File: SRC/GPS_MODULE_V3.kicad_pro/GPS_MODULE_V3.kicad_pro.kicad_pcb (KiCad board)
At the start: 4 copper layers, 50.1 x 41 mm, 127 parts, among them J3 nano_sim, J4 Micro_SD_Card, J5 Conn_02x06_Counter_Clockwise, Q1 SSM3J328R-HXY, Q2 BSN20, Q3 BSN20, U1 SY8089AAAC, U2 STM32F103C8Tx, U3 A9G_MODULE, U4 MAX485E, U5 XC6206PxxxMR, U7 ATA6561-GAQW-N, U8 W25Q32JVSS, Y1 8MHz, Y2 32.678KHz

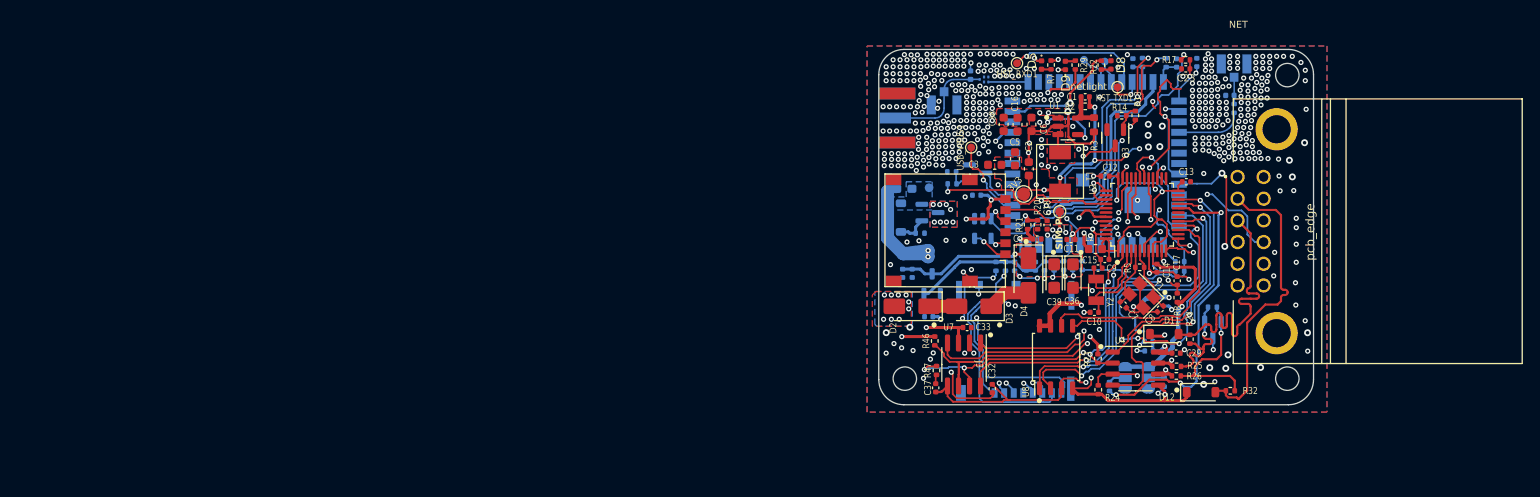
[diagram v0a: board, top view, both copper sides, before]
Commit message: GPS all files BOM and placemnt guide files added
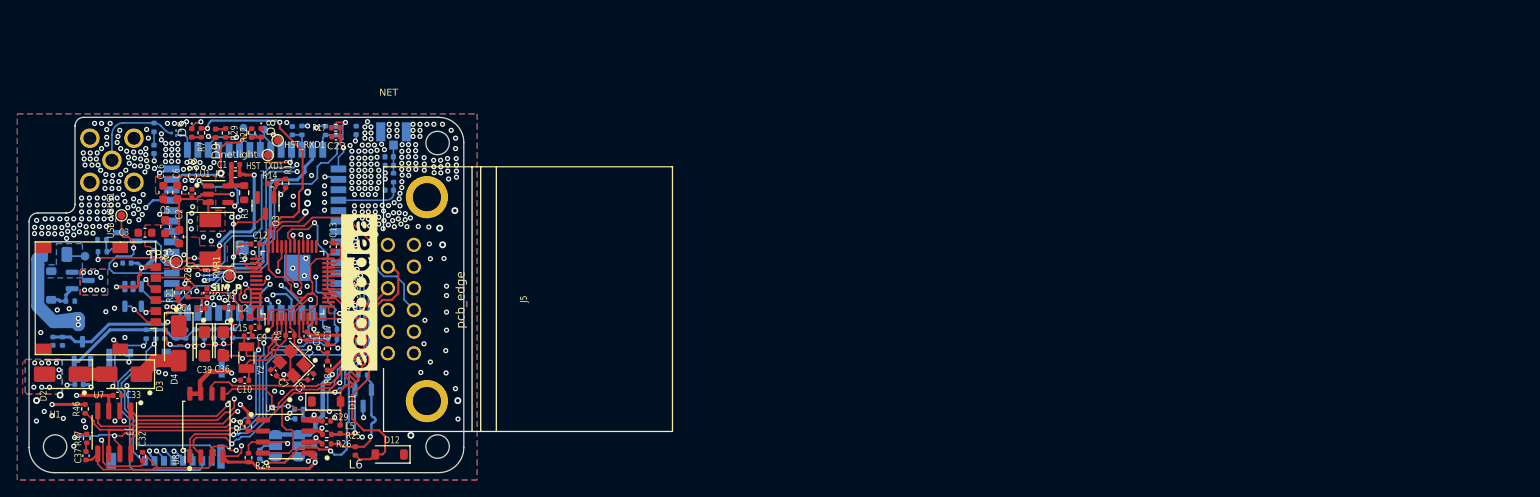
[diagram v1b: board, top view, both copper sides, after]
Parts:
- removed AE3: Antenna_Shield, greencharge-footprints:UFL_COAX_CONN23370191
- removed R32: 0R, Resistor_SMD:R_0402_1005Metric
- added C35: 100n, Capacitor_SMD:C_0402_1005Metric, B.Cu at (139.8, 89.6)
- added C40: C_Small, Capacitor_SMD:C_0402_1005Metric, B.Cu at (166.9, 82.2)
- added C41: C_Small, Capacitor_SMD:C_0402_1005Metric, B.Cu at (166.9, 79.4)
- added L5: L_Ferrite, Inductor_SMD:L_0402_1005Metric, F.Cu at (161.3, 109.8)
- added L6: L_Ferrite, Inductor_SMD:L_0402_1005Metric, F.Cu at (163.0, 112.3)
- AE1: footprint Connector_Coaxial:SMA_Samtec_SMA-J-P-X-ST-EM1_EdgeMount -> Connector_Coaxial:SMA_Molex_73251-2200_Horizontal
- C38: footprint Capacitor_SMD:C_0603_1608Metric -> Capacitor_SMD:C_0402_1005Metric
- G***: moved to F.Cu
- L2: footprint Inductor_SMD:L_0603_1608Metric -> Inductor_SMD:L_0402_1005Metric
- R28: value 0R -> 22R; moved to B.Cu
- TH1: footprint Fuse:Fuse_0603_1608Metric_Pad1.05x0.95mm_HandSolder -> Fuse:Fuse_1206_3216Metric
- TP2: footprint TestPoint:TestPoint_Pad_D1.5mm -> TestPoint:TestPoint_Pad_D1.0mm
- moved R28 121.8 mm to (139.8, 75.0)
- moved C16 98.8 mm to (140.9, 82.5)
- moved C6 98.8 mm to (142.5, 82.5)
- moved G*** 98.7 mm to (163.5, 94.0)
- moved C13 98.6 mm to (160.5, 88.7), turned to 90 degrees
- moved C23 98.2 mm to (160.8, 76.1)
- moved D10 98.2 mm to (163.9, 106.2)
- moved J5 98.2 mm to (182.4, 94.8)
- moved C12 98.2 mm to (151.5, 88.4)
- moved C14 98.2 mm to (157.5, 99.0)
- moved C15 98.2 mm to (151.5, 98.0)
- moved C17 98.2 mm to (159.8, 100.5)
- moved C19 98.2 mm to (136.7, 90.6)
- moved C24 98.2 mm to (128.2, 99.6)
- moved C26 98.2 mm to (131.2, 103.5)
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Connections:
- L3 pad 1: Net-(AE1-A) -> Net-(L3-Pad1)
- R28 pad 1: Net-(D10-K-Pad1) -> Net-(L3-Pad1)
- R28 pad 2: /RS485_MAX485/B -> Net-(AE1-A)
- U3 pad 49: /STM32F103C8T6_MCU/TX2 -> /STM32F103C8T6_MCU/RX2
- U3 pad 50: /STM32F103C8T6_MCU/RX2 -> /STM32F103C8T6_MCU/TX2
- U4 pad 1: /STM32F103C8T6_MCU/TX3 -> /STM32F103C8T6_MCU/RX3
- U4 pad 4: /STM32F103C8T6_MCU/RX3 -> /STM32F103C8T6_MCU/TX3
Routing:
- net /STM32F103C8T6_MCU/TX1: track 59.9 -> 18.0 mm
- net 2V8: track 21.0 -> 40.5 mm, vias 0 -> 2
- net +3V3: track 118.9 -> 104.1 mm, vias 13 -> 8
- net Net-(U3-HST_TXD): track 15.6 -> 3.23 mm
- net /STM32F103C8T6_MCU/TX2: track 40.2 -> 27.9 mm, vias 3 -> 2
- net Net-(D5-K): track 39.8 -> 31.0 mm
- net /STM32F103C8T6_MCU/TX3: track 27.6 -> 35.5 mm
- net Net-(U3-VUSB_DET): track 9.54 -> 16.6 mm
- net /STM32F103C8T6_MCU/RX3: track 35.8 -> 28.7 mm
- net 4.2V_SIMPWR: track 59.1 -> 52.7 mm
- net /A9G_GSM_GPRS_MODULE/TF_CARD_CONN/SD_CLK: track 44.5 -> 49.8 mm
- net GND: track 109.2 -> 104.2 mm, vias 495 -> 382
- net Net-(D10-K-Pad2): track 18.1 -> 13.3 mm
- net /A9G_GSM_GPRS_MODULE/TF_CARD_CONN/SD_D3: track 35.6 -> 39.8 mm
- net /A9G_GSM_GPRS_MODULE/TF_CARD_CONN/SD_D1: track 46.7 -> 50.7 mm
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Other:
- outline, holes or cut-outs redrawn
